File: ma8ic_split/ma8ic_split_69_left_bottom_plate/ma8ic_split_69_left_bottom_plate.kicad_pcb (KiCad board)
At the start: 2 copper layers, 166.3 x 125.7 mm, 9 parts

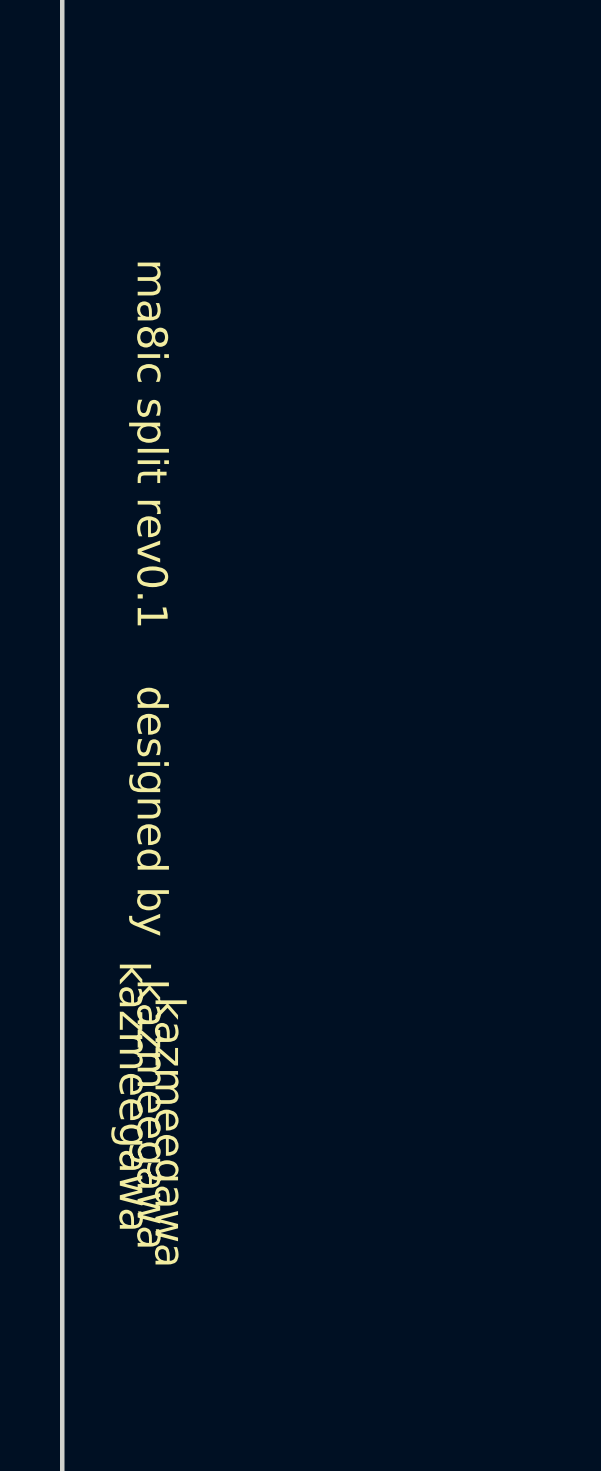
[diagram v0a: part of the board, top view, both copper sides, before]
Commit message: update
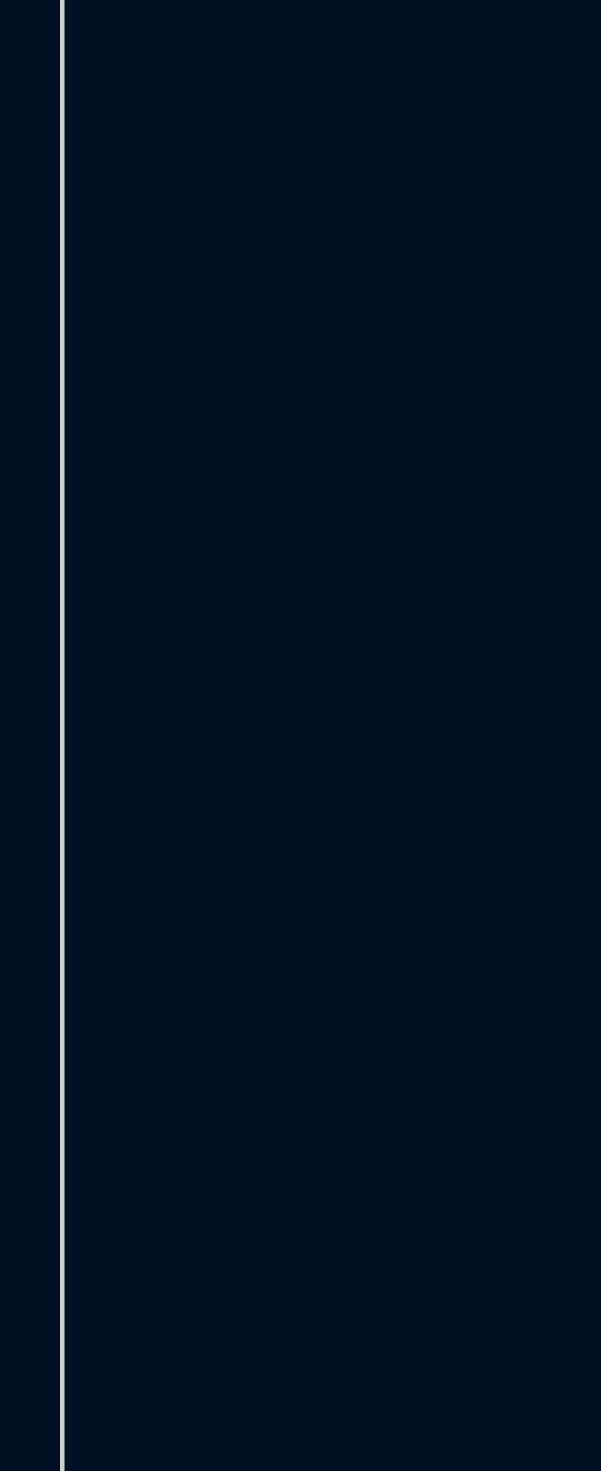
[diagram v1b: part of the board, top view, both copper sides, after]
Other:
- board text removed: "designed by"
- board text removed: "kazmeegawa"
- board text removed: "ma8ic split rev0.1"
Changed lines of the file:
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@@
     )
     (pad_to_mask_clearance 0)
-    (aux_axis_origin 59.5313 41.67191)
+    (aux_axis_origin 50.006292 32.146875)
     (pcbplotparams
       (layerselection 0x00010fc_ffffffff)
@@
     (effects (font (size 6 6) (thickness 0.8)) (justify mirror))
   )
-  (gr_text "kazmeegawa" (at 50.006392 96.432687 270) (layer "F.SilkS")
-    (effects (font (size 1 1) (thickness 0.15)))
-  )
-  (gr_text "kazmeegawa" (at 50.601705 97.028 270) (layer "F.SilkS")
-    (effects (font (size 1 1) (thickness 0.15)))
-  )
-  (gr_text "ma8ic split rev0.1" (at 50.601705 74.676 270) (layer "F.SilkS")
-    (effects (font (size 1 1) (thickness 0.15)))
-  )
-  (gr_text "kazmeegawa" (at 51.197018 97.623313 270) (layer "F.SilkS")
-    (effects (font (size 1 1) (thickness 0.15)))
-  )
-  (gr_text "designed by" (at 50.601705 86.915778 270) (layer "F.SilkS")
-    (effects (font (size 1 1) (thickness 0.15)))
-  )
-  (target plus (at 59.5313 41.67191) (size 5) (width 0.1) (layer "Edge.Cuts"))
-  (target plus (at 59.5313 41.67191) (size 5) (width 0.1) (layer "Edge.Cuts"))
+  (target plus (at 50.00625 32.146875) (size 5) (width 0.1) (layer "Edge.Cuts"))
 )

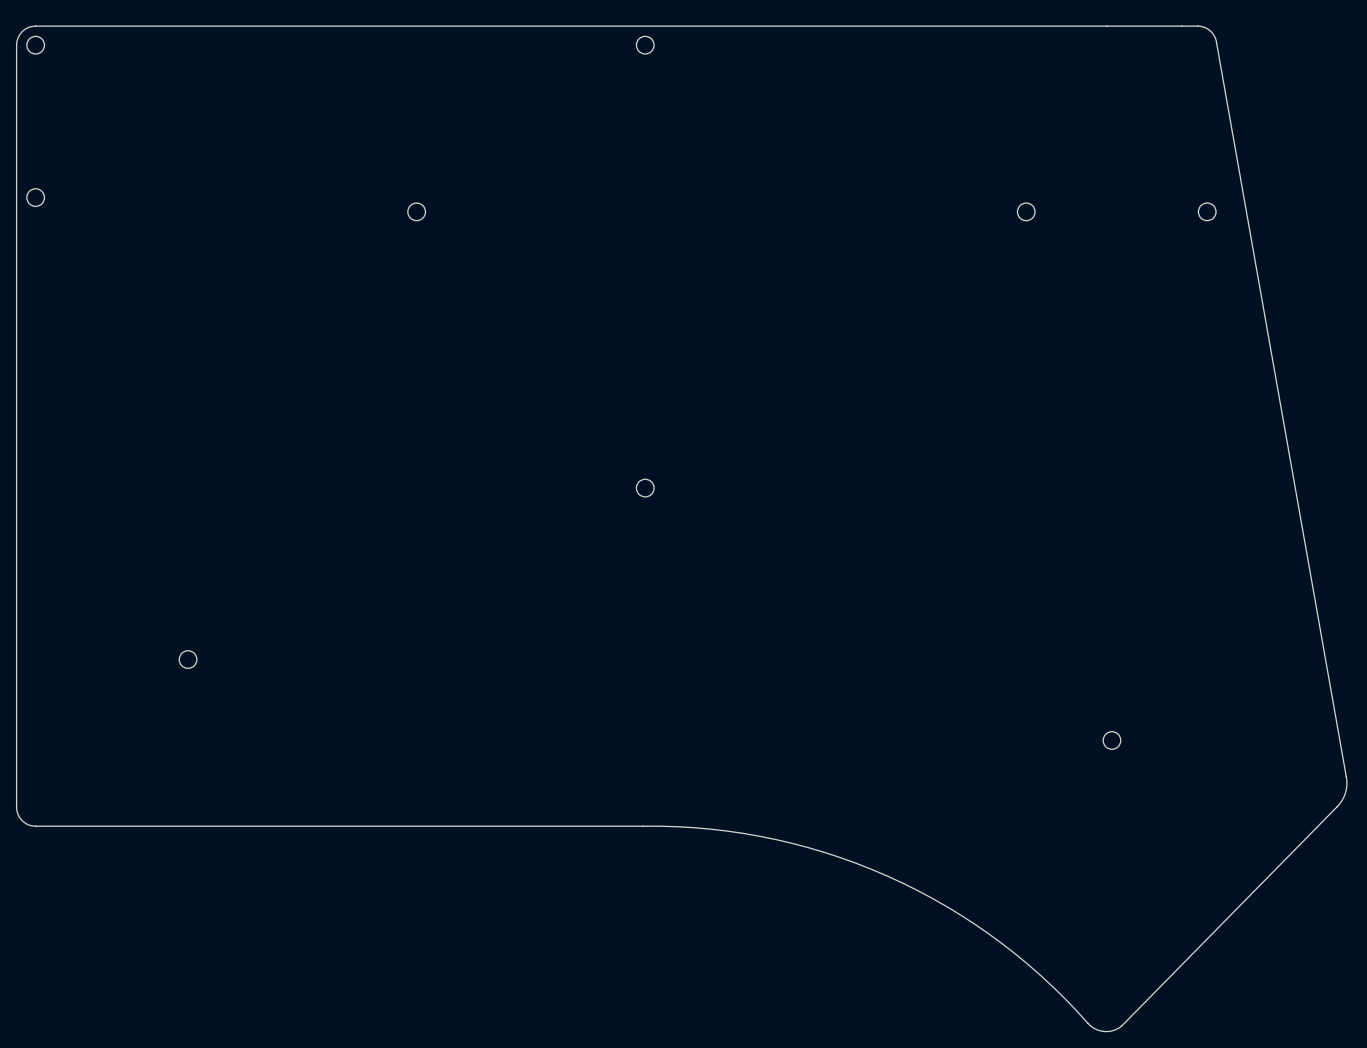
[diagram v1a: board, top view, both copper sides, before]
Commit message: update
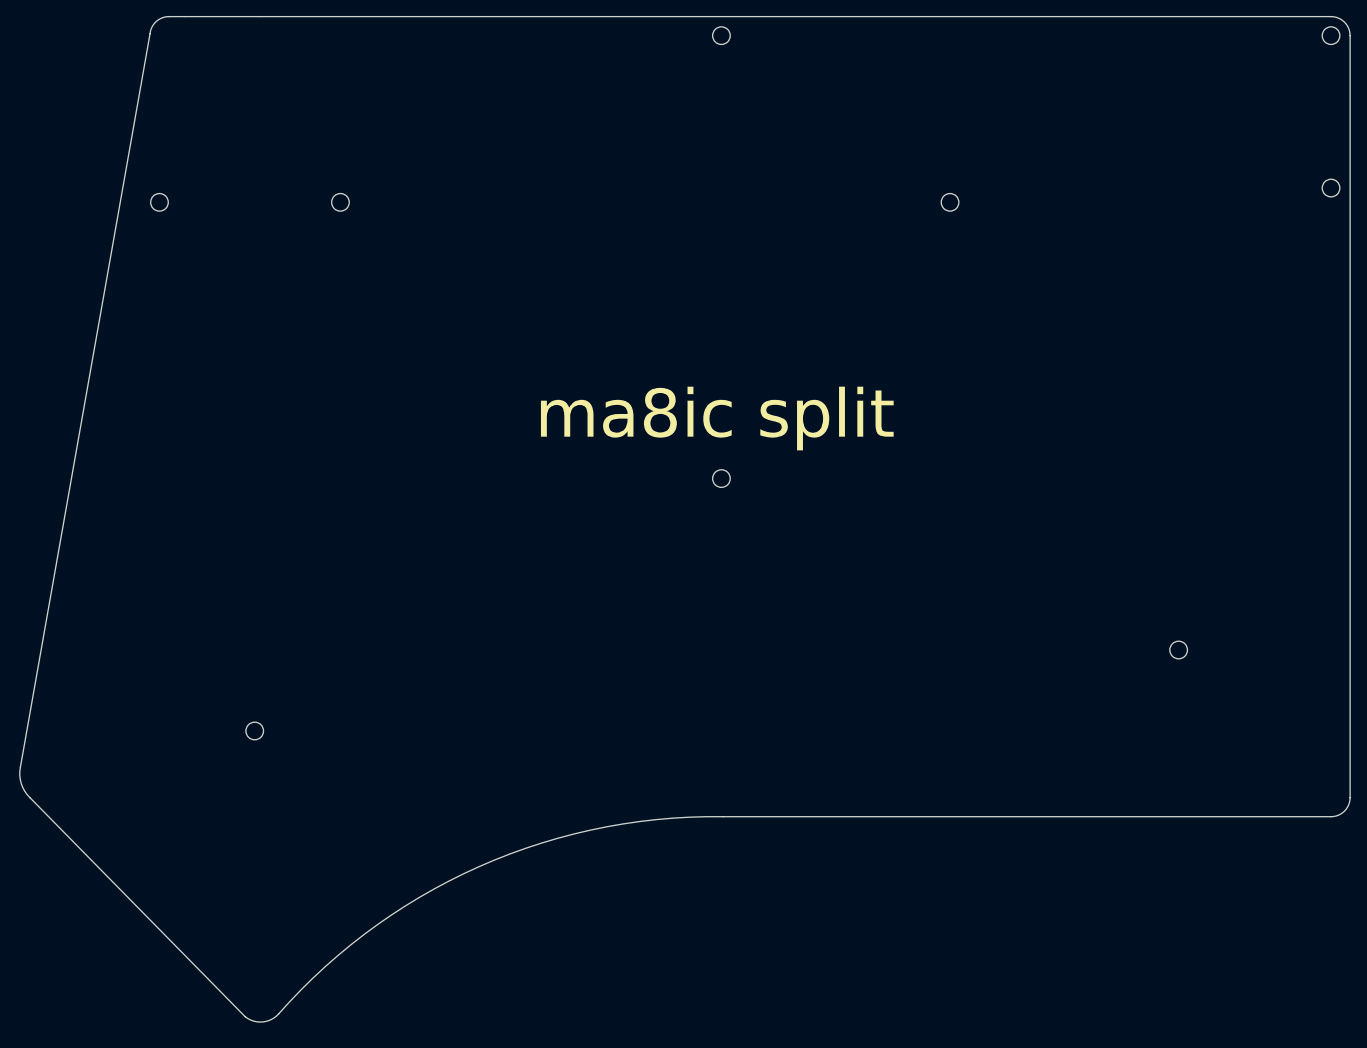
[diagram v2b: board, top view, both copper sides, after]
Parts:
- ? (x5), REF** (x4): moved to B.Cu
- moved ? 161.9 mm to (211.9, 31.0), turned to 180 degrees
- moved ? 161.9 mm to (211.9, 50.0), turned to 180 degrees
- moved ? 131.0 mm to (65.5, 51.8), turned to 180 degrees
- moved REF** 123.8 mm to (192.9, 107.8), turned to 180 degrees
- moved REF** 107.2 mm to (77.4, 117.9), turned to 180 degrees
- moved REF** 85.7 mm to (88.1, 51.8), turned to 180 degrees
- moved REF** 66.7 mm to (164.3, 51.8), turned to 180 degrees
- moved ? 9.60 mm to (135.7, 31.0), turned to 180 degrees
- moved ? 9.60 mm to (135.7, 86.3), turned to 180 degrees
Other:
- outline, holes or cut-outs redrawn
